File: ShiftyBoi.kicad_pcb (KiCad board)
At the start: 2 copper layers, 176.8 x 126.5 mm, 114 parts, among them J1 Screw_Terminal_01x08, J2 Screw_Terminal_01x08, J3 Screw_Terminal_01x08, J4 Screw_Terminal_01x08, J5 Screw_Terminal_01x08, J6 PROG, J7 Barrel_Jack_MountingPin, Q1 AO3400A, Q10 AO3400A, Q11 AO3400A, Q12 AO3400A, Q13 AO3400A, Q14 AO3400A, Q15 AO3400A, Q16 AO3400A, Q17 AO3400A, Q18 AO3400A, Q19 AO3400A, Q2 AO3400A, Q20 AO3400A, Q21 AO3400A, Q22 AO3400A, Q23 AO3400A, Q24 AO3400A, Q25 AO3400A, Q26 AO3400A, Q27 AO3400A, Q28 AO3400A, Q29 AO3400A, Q3 AO3400A, Q30 AO3400A, Q31 AO3400A, Q32 AO3400A, Q4 AO3400A, Q5 AO3400A, Q6 AO3400A, Q7 AO3400A, Q8 AO3400A, Q9 AO3400A, U1 ESP-12F, U2 74HC595, U3 74HC595, U4 74HC595, U5 74HC595, U6 AMS1117-3.3

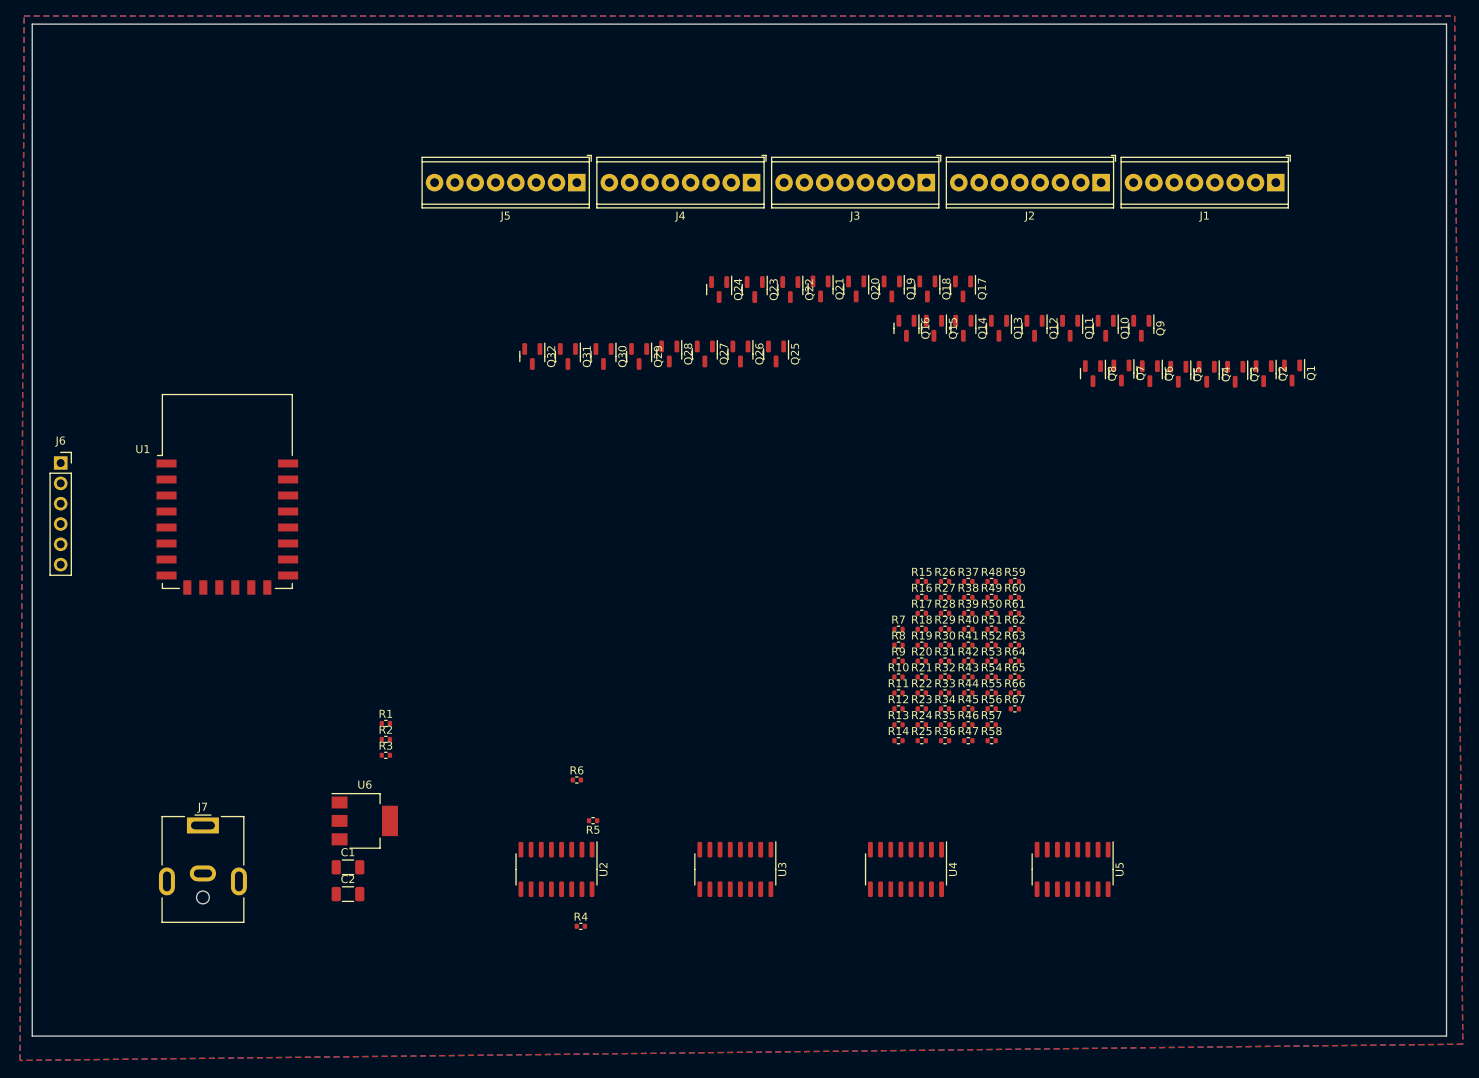
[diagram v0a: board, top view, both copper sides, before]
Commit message: More pcb layout
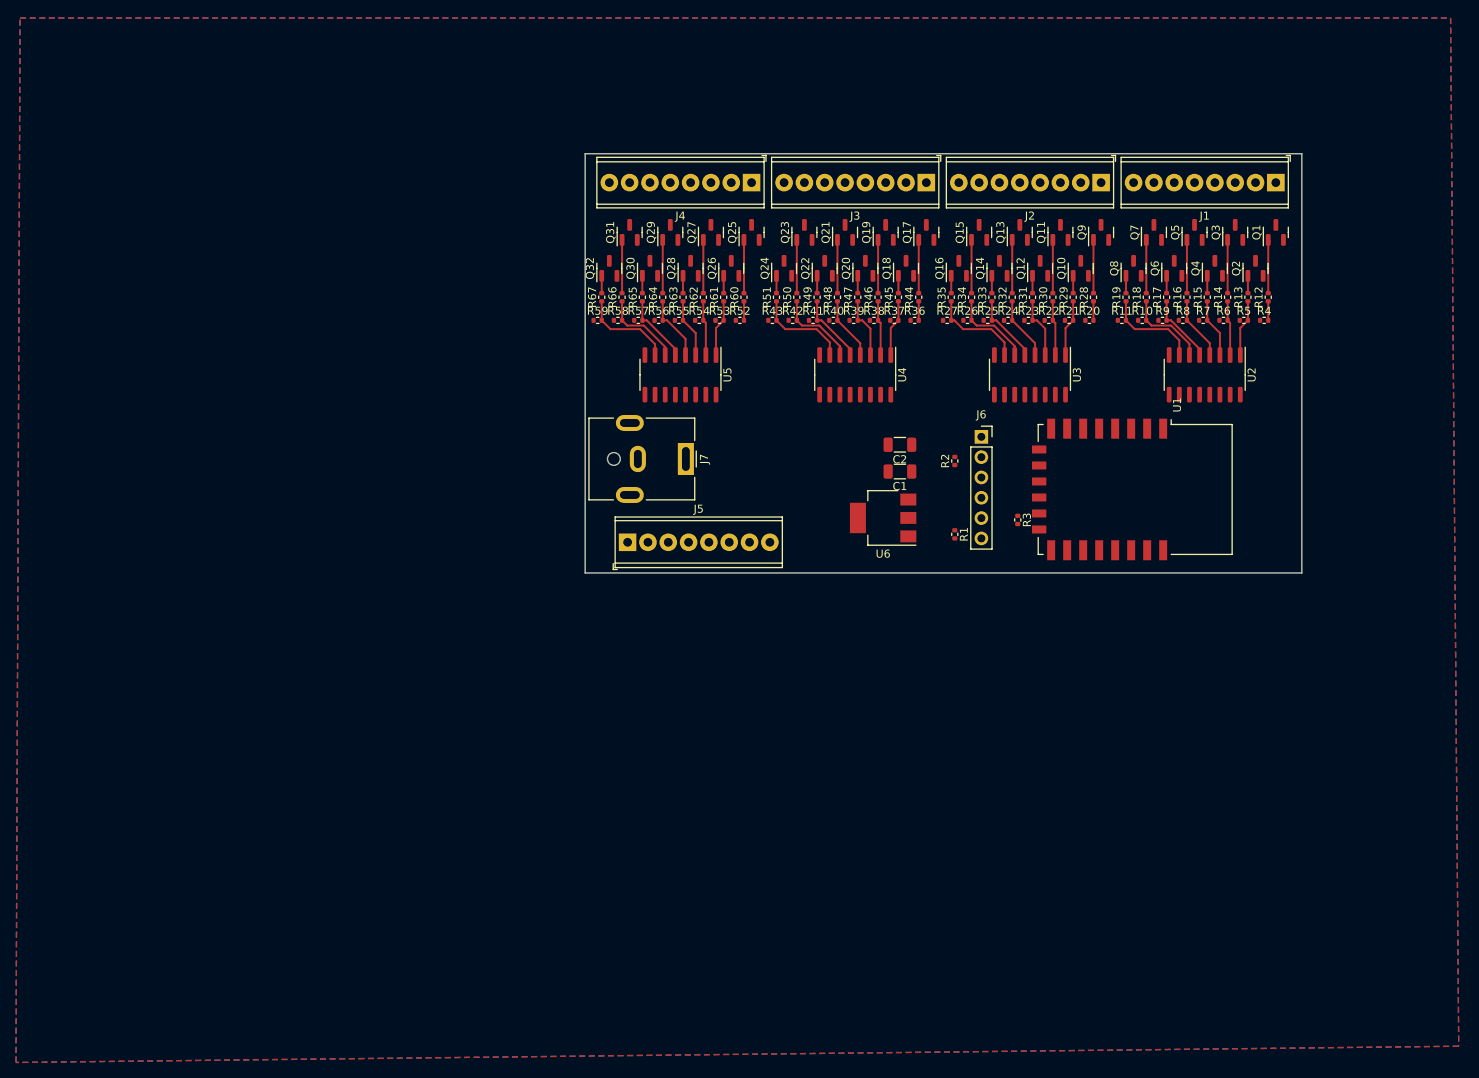
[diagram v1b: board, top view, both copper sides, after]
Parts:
- moved J6 115.1 mm to (152.2, 77.5)
- moved R4 114.2 mm to (187.5, 62.9)
- moved U1 113.5 mm to (171.4, 84.1), turned to -90 degrees
- moved R5 102.6 mm to (185.0, 62.9), turned to 0 degrees
- moved U2 101.9 mm to (180.1, 69.7)
- moved R6 99.2 mm to (182.4, 62.9)
- moved C2 89.0 mm to (142.0, 78.5), turned to 180 degrees
- moved C1 84.9 mm to (142.0, 81.8), turned to 180 degrees
- moved R3 84.3 mm to (156.7, 87.9), turned to -90 degrees
- moved R2 79.2 mm to (148.8, 80.5), turned to 90 degrees
- moved U5 78.9 mm to (114.6, 69.7)
- moved J7 75.8 mm to (115.2, 80.3), turned to -90 degrees
- moved U6 75.0 mm to (139.9, 87.6), turned to 180 degrees
- moved R1 74.9 mm to (148.8, 89.7), turned to -90 degrees
- moved R67 72.9 mm to (104.7, 60.0), turned to 90 degrees
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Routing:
- net /Driver8: track 0.00 -> 11.9 mm
- net /Driver16: track 0.00 -> 11.8 mm
- net /Driver24: track 0.00 -> 11.8 mm
- net /Driver32: track 0.00 -> 11.6 mm
- net /Driver7: track 0.00 -> 10.4 mm
- net /Driver23: track 0.00 -> 10.2 mm
- net /Driver15: track 0.00 -> 10.2 mm
- net /Driver31: track 0.00 -> 10.2 mm
- net /Driver6: track 0.00 -> 8.75 mm
- net /Driver30: track 0.00 -> 8.75 mm
- net /Driver22: track 0.00 -> 8.75 mm
- net /Driver14: track 0.00 -> 8.75 mm
- net /Driver29: track 0.00 -> 8.22 mm
- net /Driver13: track 0.00 -> 7.90 mm
- net /Driver5: track 0.00 -> 7.90 mm
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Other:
- board size 176.8 x 126.5 mm -> 89.6 x 52.4 mm
